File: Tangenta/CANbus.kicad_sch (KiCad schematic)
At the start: 1 part

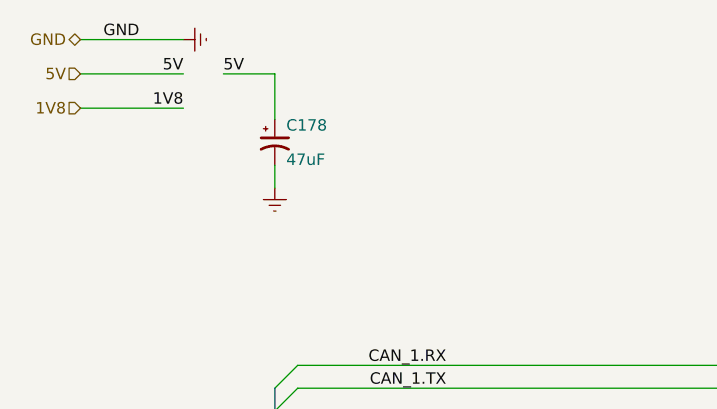
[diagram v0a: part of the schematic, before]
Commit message: initialize branch
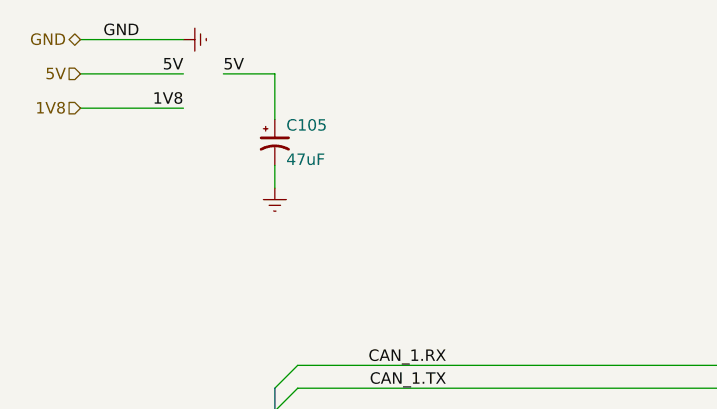
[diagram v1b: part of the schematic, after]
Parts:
- renumbered C178 to C105
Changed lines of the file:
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@@
   (symbol (lib_id "CholaSymbolsPrjLib:16CE47FSS") (at 46.99 36.83 0) (unit 1)
     (in_bom yes) (on_board yes) (dnp no)
-    (property "Reference" "C178" (at 48.26 34.925 0)
+    (property "Reference" "C105" (at 48.26 34.925 0)
       (effects (font (size 1.27 1.27)) (justify left))
     )
@@
     (instances
       (project "Tangenta"
-        (path "/358d1bcf-7599-4352-8c4d-baa18a5f09e6/2bb52479-7b35-496d-9807-27e706c6ef7b/c653b84e-94ee-4be9-b47c-8c767f88973e"
-          (reference "C178") (unit 1)
-        )
-        (path "/358d1bcf-7599-4352-8c4d-baa18a5f09e6/98e3b24f-9927-4339-b8fd-9deea91a522a"
-          (reference "C184") (unit 1)
-        )
         (path "/358d1bcf-7599-4352-8c4d-baa18a5f09e6/b5394a48-5ef8-44c9-9d56-604d4ce6d7c8"
           (reference "C105") (unit 1)
@@
   (symbol (lib_id "power:GNDREF") (at 46.99 41.91 0) (unit 1)
     (in_bom yes) (on_board yes) (dnp no) (fields_autoplaced)
-    (property "Reference" "#PWR030" (at 46.99 48.26 0)
+    (property "Reference" "#PWR060" (at 46.99 48.26 0)
       (effects (font (size 1.27 1.27)) hide)
     )
@@
     (instances
       (project "Tangenta"
-        (path "/358d1bcf-7599-4352-8c4d-baa18a5f09e6/b1871a4d-6a35-44e2-a9a2-9a4af684371d"
-          (reference "#PWR030") (unit 1)
-        )
-        (path "/358d1bcf-7599-4352-8c4d-baa18a5f09e6/f1c5822c-e7b8-40ae-bab0-71fd1c2cfc7c"
-          (reference "#PWR035") (unit 1)
-        )
-        (path "/358d1bcf-7599-4352-8c4d-baa18a5f09e6/98e3b24f-9927-4339-b8fd-9deea91a522a"
-          (reference "#PWR081") (unit 1)
-        )
         (path "/358d1bcf-7599-4352-8c4d-baa18a5f09e6/b5394a48-5ef8-44c9-9d56-604d4ce6d7c8"
           (reference "#PWR060") (unit 1)
@@
   (symbol (lib_id "power:GNDREF") (at 36.83 25.4 90) (unit 1)
     (in_bom yes) (on_board yes) (dnp no) (fields_autoplaced)
-    (property "Reference" "#PWR030" (at 43.18 25.4 0)
+    (property "Reference" "#PWR059" (at 43.18 25.4 0)
       (effects (font (size 1.27 1.27)) hide)
     )
@@
     (instances
       (project "Tangenta"
-        (path "/358d1bcf-7599-4352-8c4d-baa18a5f09e6/b1871a4d-6a35-44e2-a9a2-9a4af684371d"
-          (reference "#PWR030") (unit 1)
-        )
-        (path "/358d1bcf-7599-4352-8c4d-baa18a5f09e6/f1c5822c-e7b8-40ae-bab0-71fd1c2cfc7c"
-          (reference "#PWR035") (unit 1)
-        )
-        (path "/358d1bcf-7599-4352-8c4d-baa18a5f09e6/98e3b24f-9927-4339-b8fd-9deea91a522a"
-          (reference "#PWR076") (unit 1)
-        )
         (path "/358d1bcf-7599-4352-8c4d-baa18a5f09e6/b5394a48-5ef8-44c9-9d56-604d4ce6d7c8"
           (reference "#PWR059") (unit 1)
